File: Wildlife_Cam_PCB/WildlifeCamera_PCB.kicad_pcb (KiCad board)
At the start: 2 copper layers, 39.9 x 79.9 mm, 36 parts, among them J1 PIR, J10 POWER, J2 TRIG, J3 RTC_DS3231, J4 PROG, J5 PROG_EN, J6 LOGO1, J7 LOGO2, J8 PCB, Q1 2N3904, Q2 2N3904, Q3 BD135, SW1 POWER, SW2 TRIGGER, U1 MCP1826S-3302, U3 ESP32_CAM

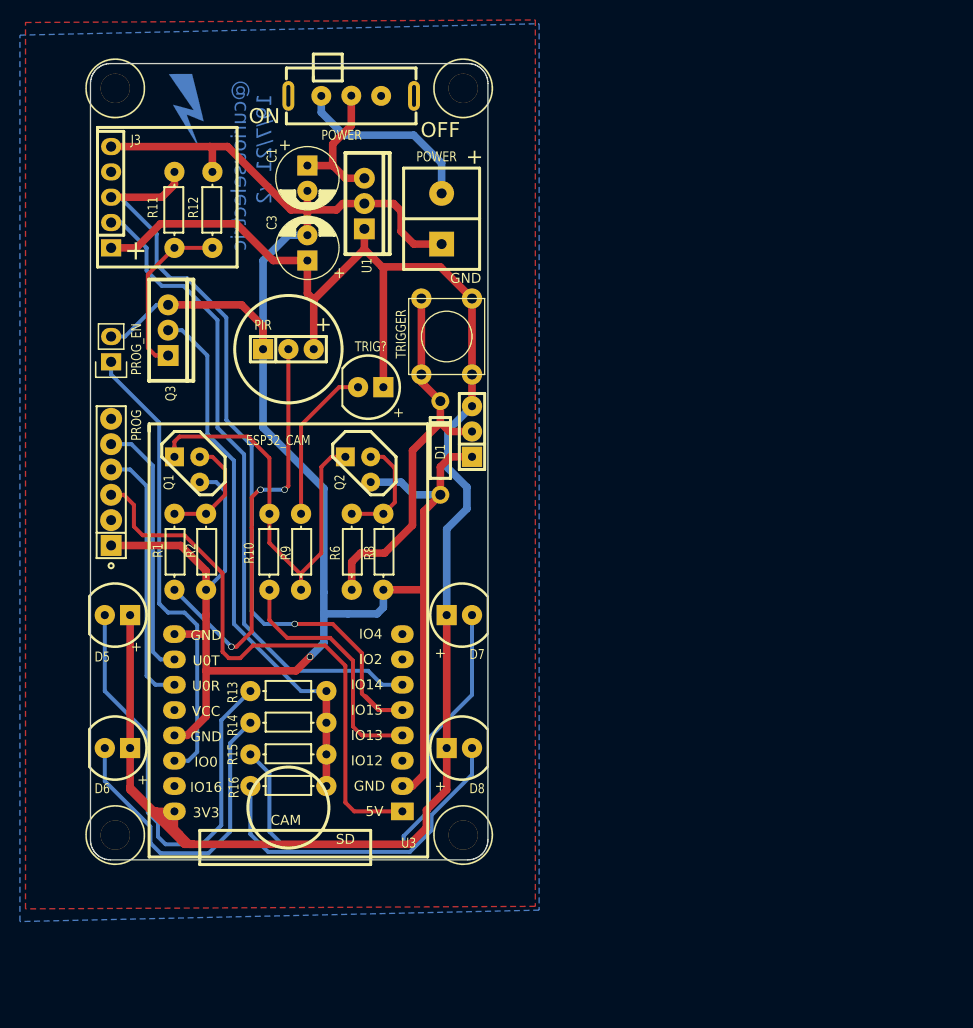
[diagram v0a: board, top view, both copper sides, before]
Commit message: Small updates to PCB
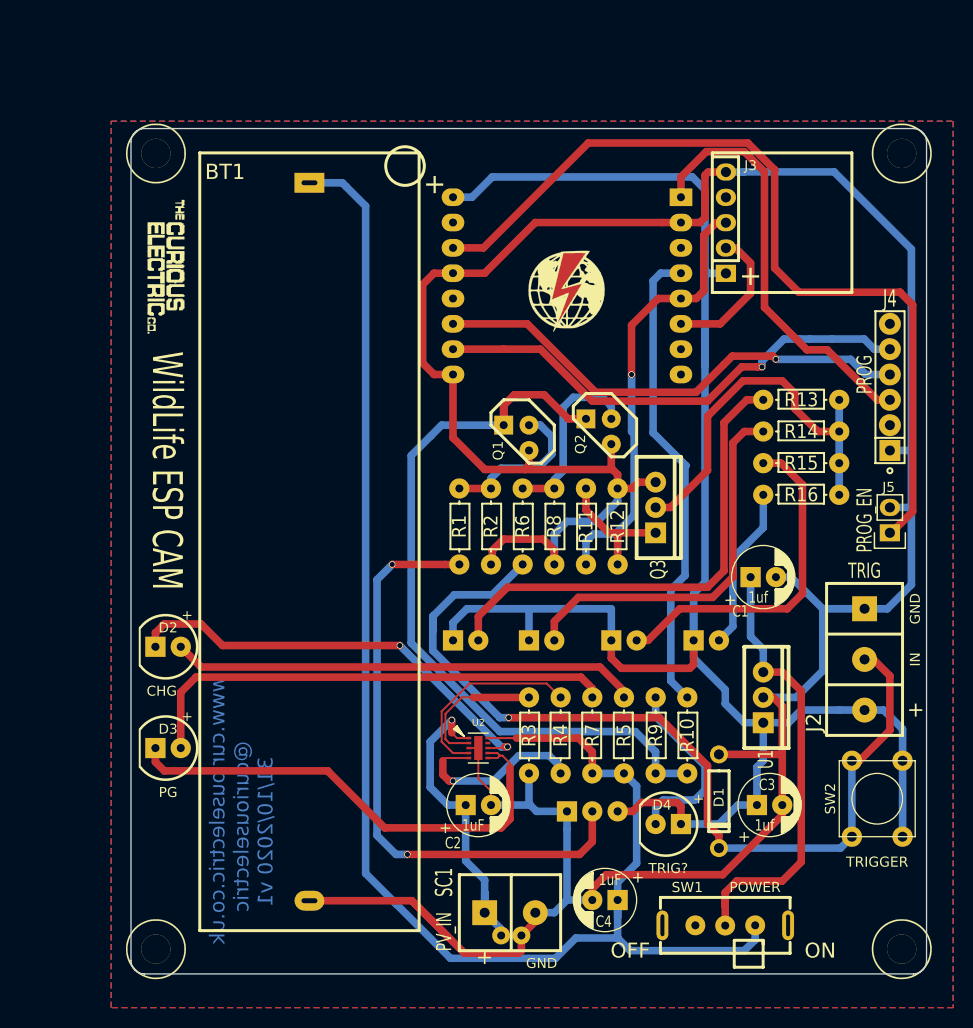
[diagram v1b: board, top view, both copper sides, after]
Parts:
- removed J10: POWER, REInnovationFootprint:SIL-2_screw_terminal
- added BT1: 18650 LiIon Cell, REInnovationFootprint:TH_LiIon_Holder, F.Cu at (111.1, 55.9)
- added C2: 1uF, REInnovationFootprint:C_1V7_TH, F.Cu at (139.1, 121.3)
- added C4: 1uF, REInnovationFootprint:C_1V7_TH, F.Cu at (151.8, 130.8)
- added D2: CHG, REInnovationFootprint:TH_LED-5MM_larg_pad, F.Cu at (108.0, 105.4)
- added D3: PG, REInnovationFootprint:TH_LED-5MM_larg_pad, F.Cu at (108.0, 115.6)
- added R3: 1k, REInnovationFootprint:TH_Resistor_1, F.Cu at (144.1, 114.3)
- added R4: 100k, REInnovationFootprint:TH_Resistor_1, F.Cu at (147.3, 114.3)
- added R5: 2.2k, REInnovationFootprint:TH_Resistor_1, F.Cu at (153.7, 114.3)
- added R7: 2.2k, REInnovationFootprint:TH_Resistor_1, F.Cu at (150.5, 114.3)
- added SC1: PV_IN, REInnovationFootprint:SIL_2_screw_+_JST_2mm, F.Cu at (139.7, 132.1)
- added U2: BQ24210, REInnovationFootprint:SM_WSON-10-2x3, F.Cu at (139.1, 115.6)
- D5, D6, D7, D8, J1, J7: moved to B.Cu
- J2: footprint REInnovationFootprint:SIL-3_lg_pad -> REInnovationFootprint:SIL-3_screw_terminal
- J6, U3: moved to F.Cu
- J8: footprint REInnovationFootprint:PCB_SolarChargerPCB40x80 -> REInnovationFootprint:PCB_Wildlife_Cam
- moved J8 97.1 mm to (198.8, 146.1)
- moved SW1 91.3 mm to (163.8, 133.3), turned to 270 degrees
- moved J5 80.0 mm to (180.3, 94.0)
- moved J4 78.7 mm to (180.3, 79.4)
- moved C3 72.6 mm to (168.3, 121.3), turned to 0 degrees
- moved U3 67.6 mm to (148.0, 60.3)
- moved U1 63.7 mm to (167.6, 110.5)
- moved SW2 63.4 mm to (179.1, 120.7)
- moved J3 61.7 mm to (176.5, 55.9)
- moved C1 60.8 mm to (167.6, 98.4), turned to 0 degrees
- moved R13 59.2 mm to (171.4, 80.6)
- moved R14 59.2 mm to (171.4, 83.8)
- moved R15 59.2 mm to (171.4, 87.0)
- moved R16 59.2 mm to (171.4, 90.2)
- moved J1 55.5 mm to (150.5, 121.9)
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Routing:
- net VCC: track 18.9 -> 155.9 mm
- net GND: track 228.5 -> 303.6 mm, vias 1 -> 0
- net Net-(D3-Pad1): track 0.00 -> 62.9 mm
- net Net-(D1-Pad1): track 38.6 -> 92.4 mm, vias 0 -> 1
- net /I2C_DAT: track 66.0 -> 14.4 mm
- net Net-(D3-Pad2): track 0.00 -> 48.9 mm
- net Net-(D2-Pad2): track 0.00 -> 46.9 mm
- net Net-(D2-Pad1): track 0.00 -> 44.2 mm, vias 0 -> 2
- net /PROG_EN: track 46.3 -> 86.8 mm
- net /I2C_CLK: track 82.9 -> 44.4 mm
- net /TRIG: track 43.7 -> 76.7 mm
- net Net-(C1-Pad1): track 14.0 -> 44.7 mm
- net Net-(C2-Pad1): track 0.00 -> 30.4 mm, vias 0 -> 1
- net Net-(Q3-Pad2): track 64.1 -> 39.4 mm
- net /U0T: track 26.2 -> 49.3 mm, vias 0 -> 1
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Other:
- board size 39.9 x 79.9 mm -> 79.8 x 84.8 mm
- board text added: "31/10/2020 v1"
- board text added: "FLASH"
- board text added: "WildLife ESP CAM"
- board text removed: "19/7/21 v2"
- board text removed: "LAPSE-O-MATIC"
